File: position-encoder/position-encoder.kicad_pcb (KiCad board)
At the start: 2 copper layers, 65 x 15 mm, 11 parts, among them J1 Conn_01x04_Male, U1 TLE4905L, U2 TLE4905L

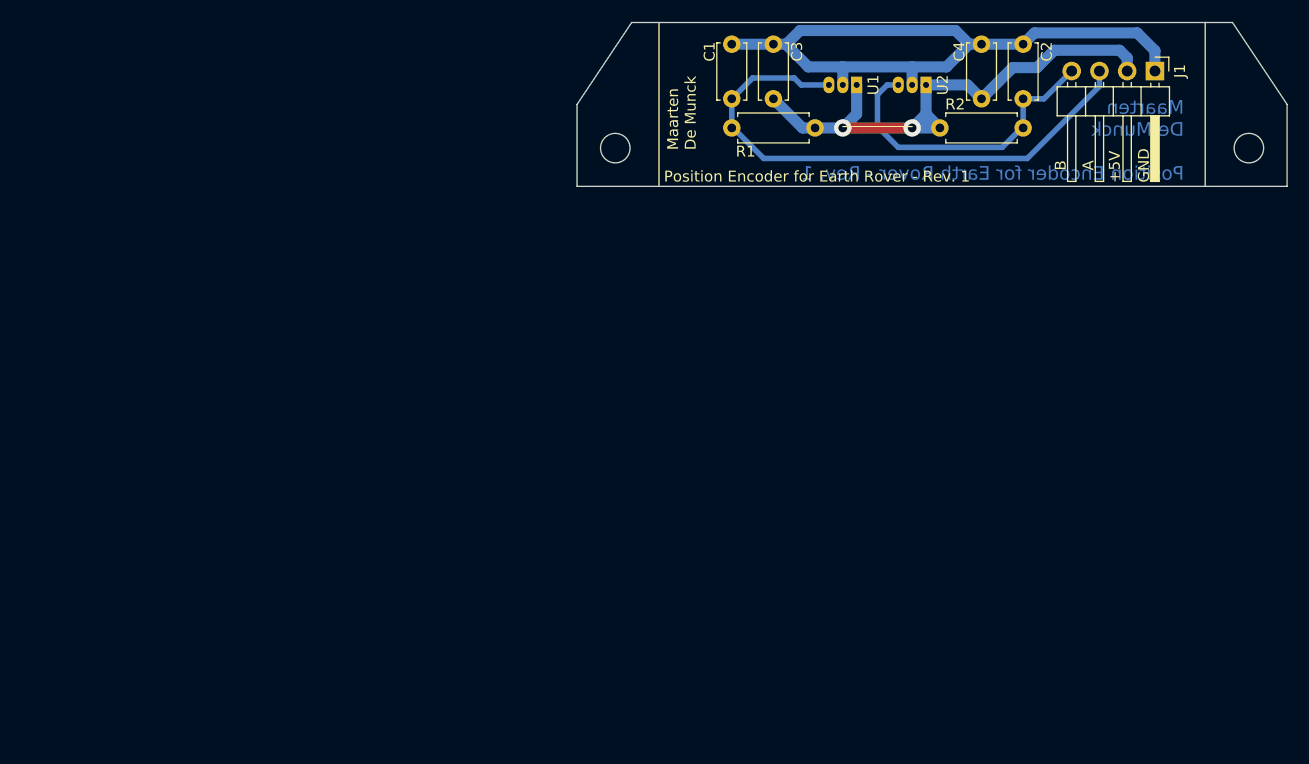
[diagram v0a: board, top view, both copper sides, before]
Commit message: Improve PCB
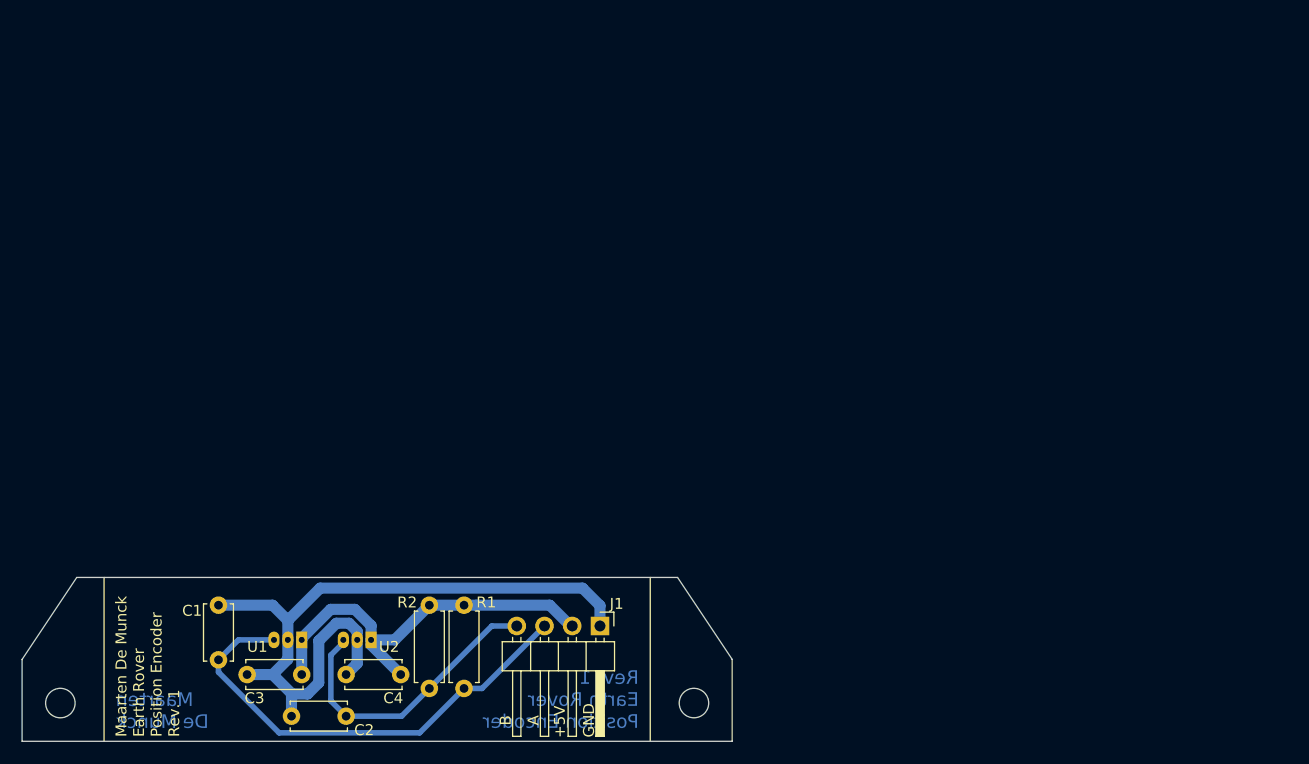
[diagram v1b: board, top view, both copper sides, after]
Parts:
- moved C2 83.9 mm to (103.8, 139.7), turned to 180 degrees
- moved C4 74.9 mm to (108.8, 135.9), turned to 180 degrees
- moved J1 71.8 mm to (127.0, 131.4)
- moved REF** 71.8 mm to (77.6, 138.5)
- moved REF** 71.8 mm to (135.6, 138.5)
- moved U1 71.8 mm to (99.7, 132.7)
- moved U2 71.8 mm to (106.0, 132.7)
- moved C1 69.6 mm to (92.1, 134.5)
- moved C3 68.1 mm to (99.7, 135.9), turned to 180 degrees
- moved R2 64.0 mm to (111.4, 129.5), turned to 270 degrees
- moved R1 54.2 mm to (114.6, 129.5), turned to 270 degrees
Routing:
- net +5V: track 49.3 -> 37.7 mm, vias 2 -> 0
- net Net-(C1-Pad1): track 51.5 -> 43.2 mm
- net GND: track 64.5 -> 67.3 mm
- net Net-(C2-Pad1): track 28.4 -> 27.1 mm
- removed copper zone on B.Cu, net GND
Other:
- net class Power added: clearance 0.254, trace_width 1.016, via_dia 1.6, via_drill 0.8
- net class Signal added: clearance 0.254, trace_width 0.508, via_dia 1.6, via_drill 0.8
- board text added: "Maarten De Munck Earth Rover Position Encoder Rev. 1"
- board text added: "Rev. 1 Earth Rover Position Encoder"
- board text removed: "Maarten De Munck Position Encoder for Earth Rover - Rev. 1"
- board text removed: "Position Encoder for Earth Rover - Rev. 1"
